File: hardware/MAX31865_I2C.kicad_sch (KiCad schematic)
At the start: 38 parts, among them J1 Conn_01x08, J2 AVR-ISP-6, J3 Conn_02x04_Odd_Even, J4 Conn_02x04_Odd_Even, J5 Conn_02x02_Odd_Even, U1 ATmega48A-A, Y1 16MHz

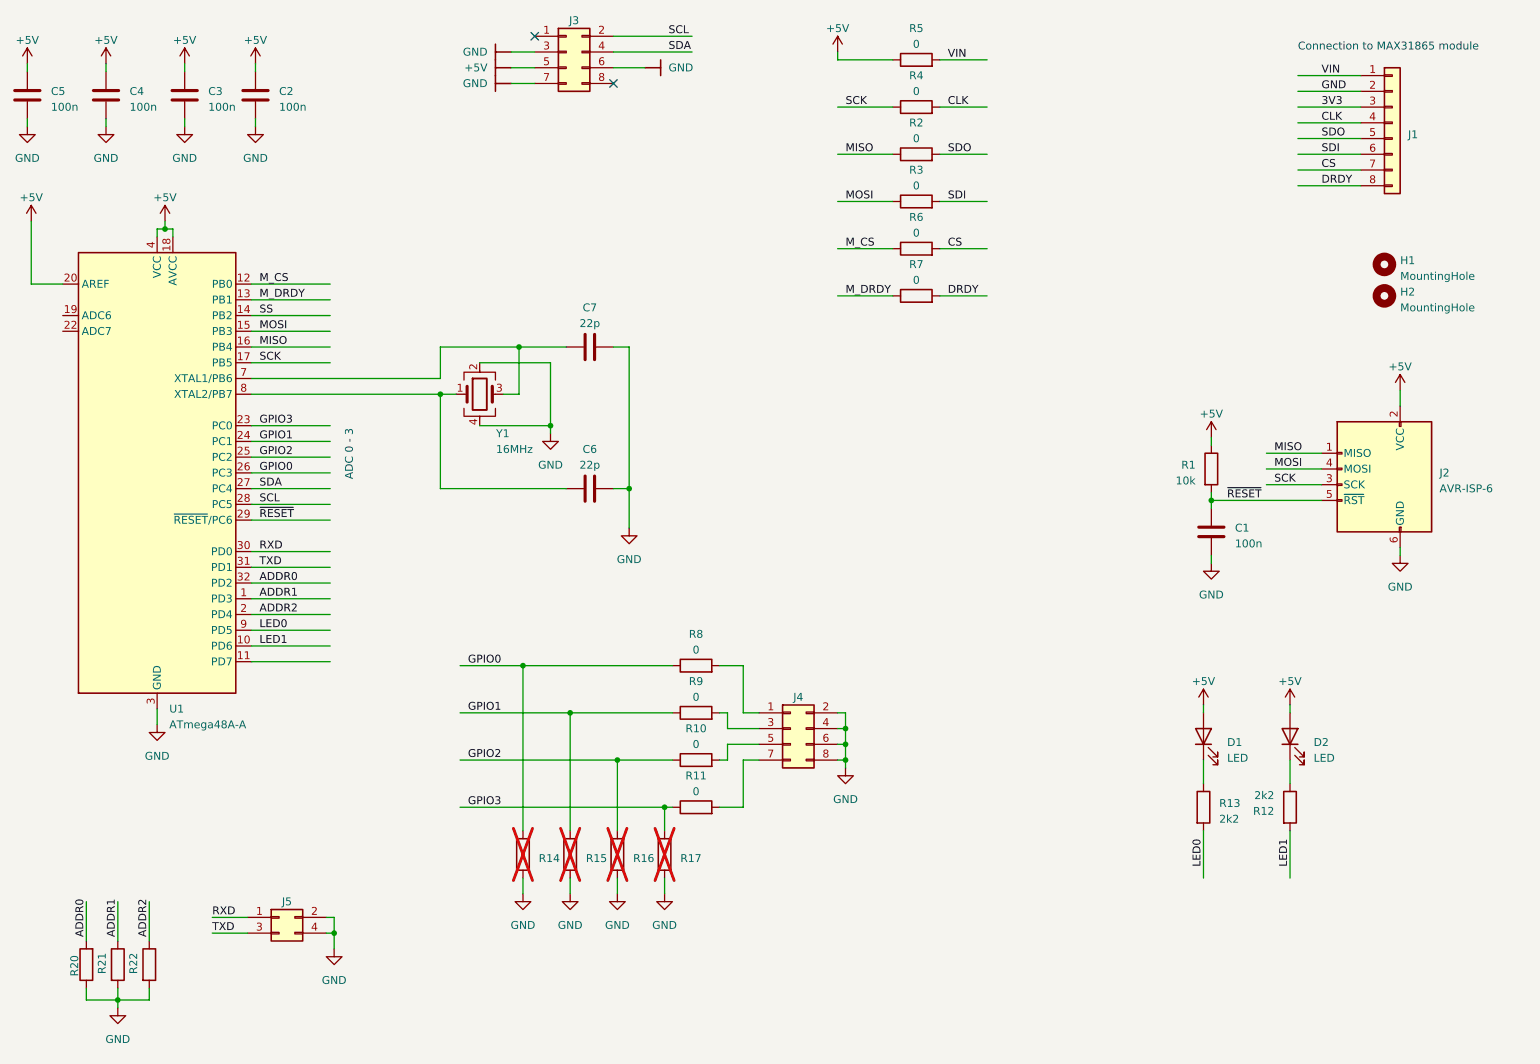
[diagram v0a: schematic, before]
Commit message: ERC and DRC clean
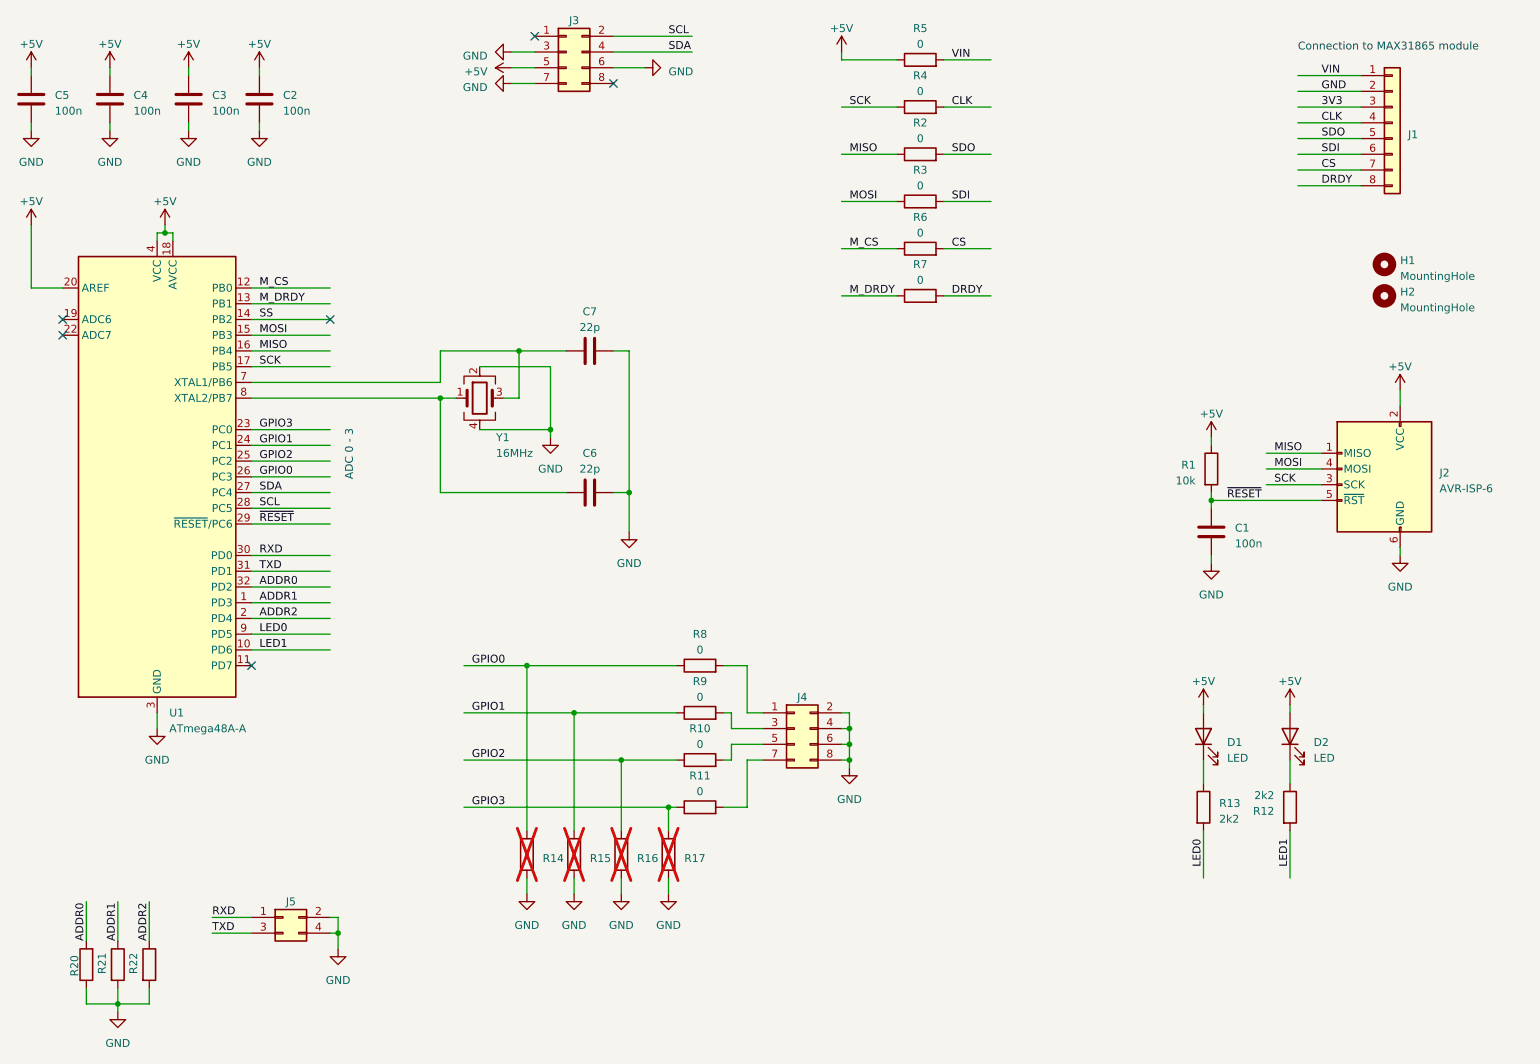
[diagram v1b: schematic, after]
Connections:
- no-connect marks 2 -> 6
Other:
- moved on the sheet: C2, C3, C4, C5, C6, C7, J4, J5, R10, R11, R14, R15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
